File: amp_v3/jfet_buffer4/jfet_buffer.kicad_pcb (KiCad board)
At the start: 2 copper layers, 37.5 x 45.1 mm, 20 parts, among them J1 SIG_OUT_L1, J2 SIG_OUT_L1, J3 SIG_OUT_L1, J4 SIG_OUT_L2, Q1 2N5457, Q2 2N5457 DSG

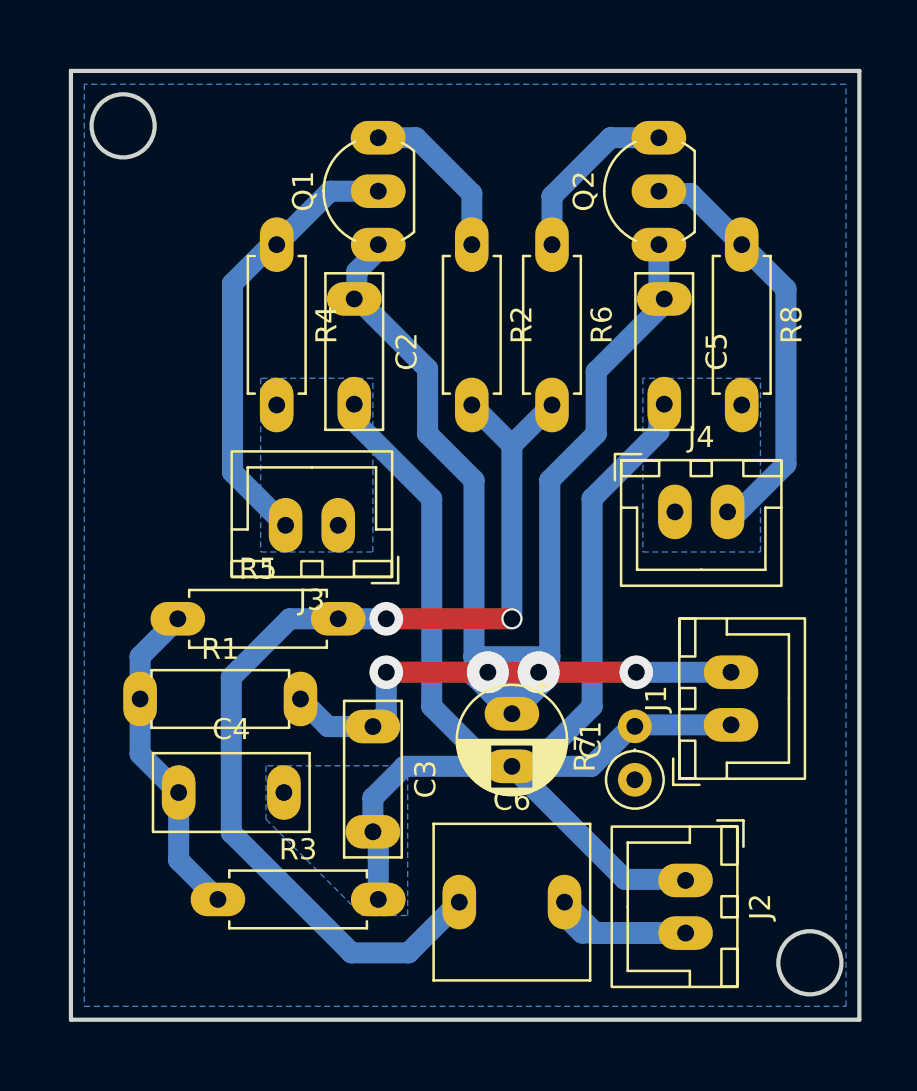
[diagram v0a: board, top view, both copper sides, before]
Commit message: update
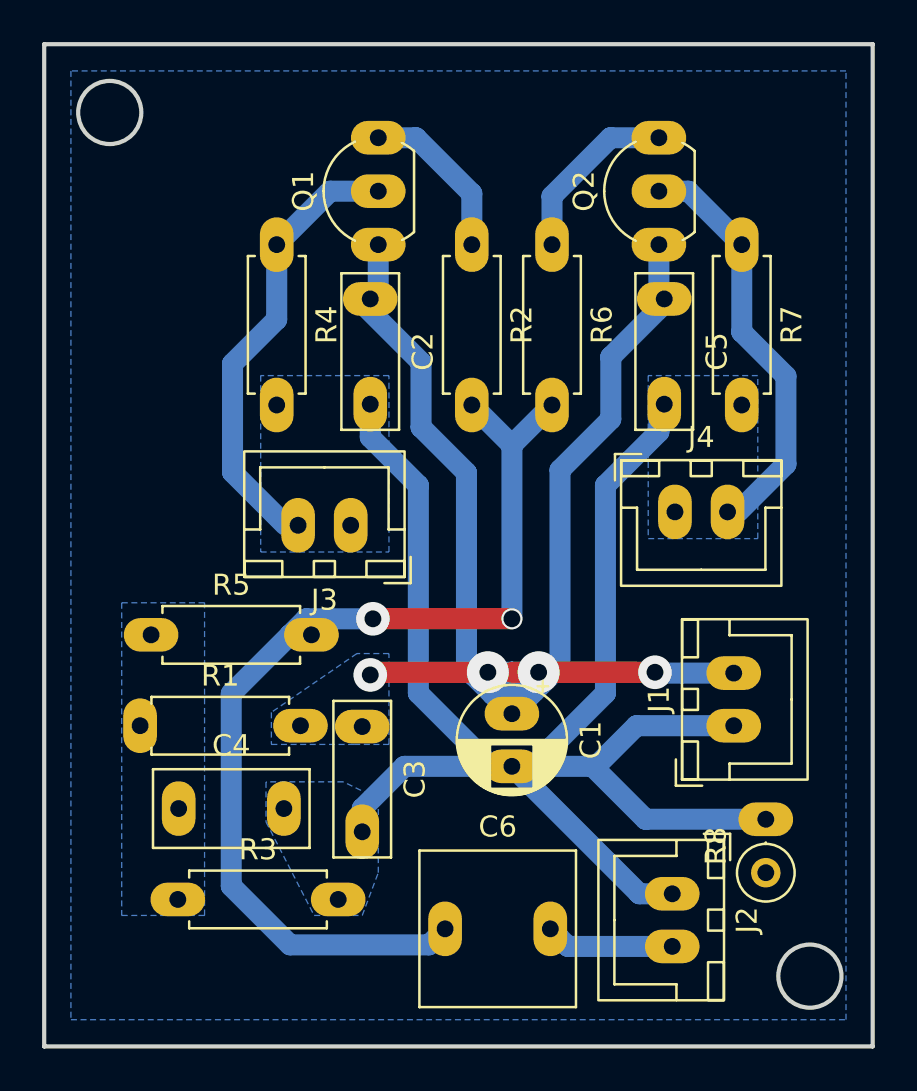
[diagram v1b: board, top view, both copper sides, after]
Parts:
- J1: value SIG_OUT_L1 -> PWR
- J2: value SIG_OUT_L1 -> INPUT
- J3: value SIG_OUT_L1 -> OUT1
- J4: value SIG_OUT_L2 -> OUT2
- Q2: value 2N5457 DSG -> 2N5457
- moved R8 7.63 mm to (103.9, 92.8)
- moved R3 1.91 mm to (75.9, 94.1)
- moved R5 1.48 mm to (74.6, 81.5)
- moved C6 1.44 mm to (88.6, 95.5)
- moved R1 1.27 mm to (74.1, 85.9)
- moved J2 0.90 mm to (99.4, 93.8)
- moved C2 0.76 mm to (85.1, 65.6)
- moved C4 0.76 mm to (76.0, 89.8)
- moved J3 0.59 mm to (84.1, 76.3)
- moved C3 0.51 mm to (84.7, 85.9)
- moved J1 0.13 mm to (102.3, 85.9)
- renumbered R8 to R7, R7 to R8
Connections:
- net /L_IN renamed /INPUT
- net /L_OUT_BUF1 renamed /OUT1
- net /L_OUT_BUF2 renamed /OUT2
- net /VBIAS_L renamed /VBIAS
- net /VBIAS_OUT_L renamed /VBIAS_OUT
- net GND_IN_L renamed GND
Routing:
- net /VBIAS: track 15.6 -> 0.00 mm
- net /INPUT: track 13.1 -> 6.14 mm
- net +20V: track 86.6 -> 82.6 mm
- net GND: track 76.1 -> 80.0 mm
- net /VBIAS_OUT: track 50.3 -> 51.3 mm
- added copper zone on B.Cu, net +20V
- added copper zone on B.Cu, net /VBIAS
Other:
- board size 37.5 x 45.1 mm -> 39.4 x 47.6 mm

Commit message: updates
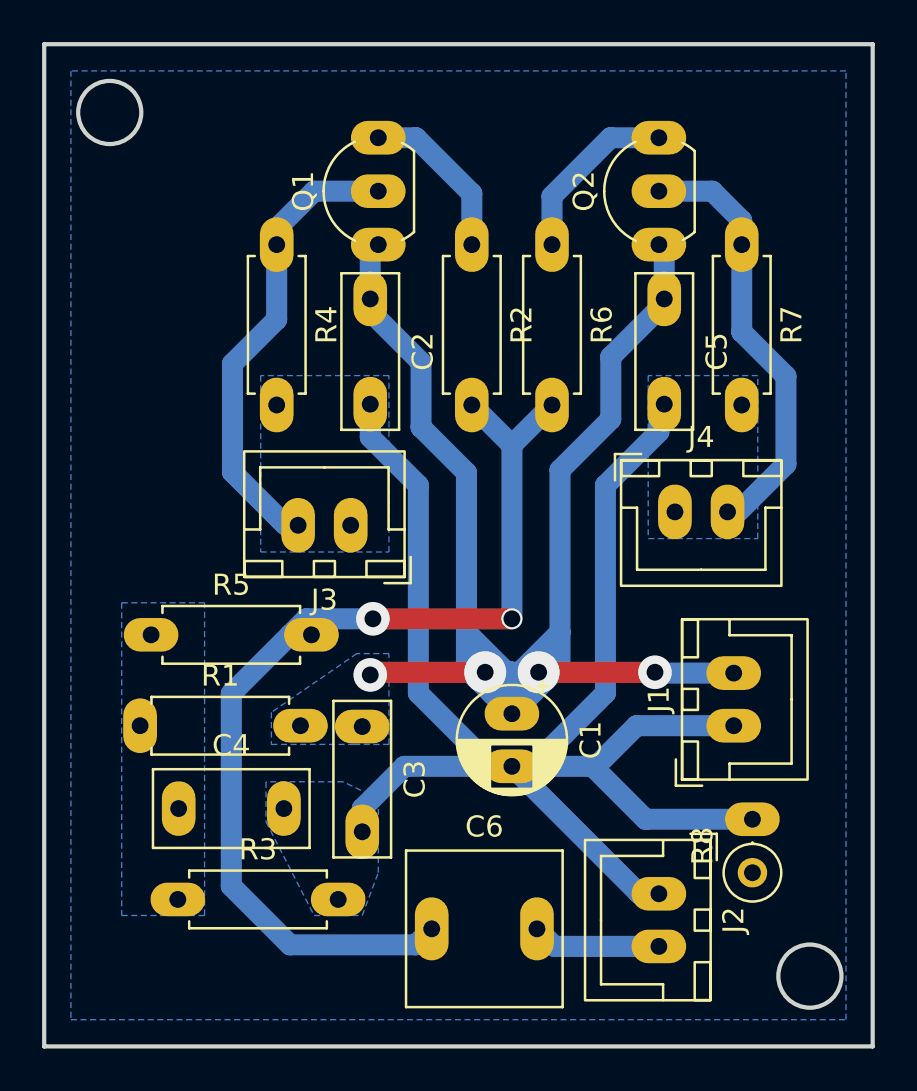
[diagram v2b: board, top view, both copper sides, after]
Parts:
- moved C6 0.64 mm to (88.0, 95.5)
- moved R8 0.64 mm to (103.2, 92.8)
- moved J2 0.63 mm to (98.8, 93.8)
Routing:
- net /VBIAS_OUT: track 51.3 -> 48.6 mm
- net +20V: track 82.6 -> 81.8 mm
- net /OUT2: track 19.5 -> 20.2 mm
- net GND: track 80.0 -> 79.4 mm
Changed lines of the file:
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@@
 	(footprint "Resistor_THT:R_Axial_DIN0207_L6.3mm_D2.5mm_P2.54mm_Vertical"
 		(layer "F.Cu")
-		(at 103.857 92.843 90)
+		(at 103.222 92.843 90)
 		(descr "Resistor, Axial_DIN0207 series, Axial, Vertical, pin pitch=2.54mm, 0.25W = 1/4W, length*diameter=6.3*2.5mm^2, http://cdn-reichelt.de/documents/datenblatt/B400/1_4W%23YAG.pdf")
 		(tags "Resistor Axial_DIN0207 series Axial Vertical pin pitch 2.54mm 0.25W = 1/4W length 6.3mm diameter 2.5mm")
@@
 		)
 		(pad "1" thru_hole oval
-			(at 0 0 270)
+			(at 0 0)
 			(size 1.6 2.6)
 			(drill 0.8)
@@
 		)
 		(pad "1" thru_hole oval
-			(at 0 0 270)
+			(at 0 0)
 			(size 1.6 2.6)
 			(drill 0.8)
@@
 	(footprint "Connector_JST:JST_XH_B2B-XH-A_1x02_P2.50mm_Vertical"
 		(layer "F.Cu")
-		(at 99.411776 93.844892 -90)
+		(at 98.777 93.844892 -90)
 		(descr "JST XH series connector, B2B-XH-A (http://www.jst-mfg.com/product/pdf/eng/eXH.pdf)")
 		(tags "connector JST XH vertical")
@@
 	(footprint "Capacitor_THT:C_Rect_L7.2mm_W7.2mm_P5.00mm_FKS2_FKP2_MKS2_MKP2"
 		(layer "F.Cu")
-		(at 88.617 95.51)
+		(at 87.982 95.51)
 		(descr "C, Rect series, Radial, pin pitch=5.00mm, length*width=7.2*7.2mm^2, Capacitor, http://www.wima.com/EN/WIMA_FKS_2.pdf")
 		(tags "C Rect series Radial pin pitch 5.00mm length 7.2mm width 7.2mm Capacitor")
@@
 		(pad "1" thru_hole oval
 			(at 0 0)
-			(size 1.6 2.6)
+			(size 1.6 3)
 			(drill 0.8)
 			(layers "*.Cu" "*.Mask")
@@
 		(pad "2" thru_hole oval
 			(at 5 0)
-			(size 1.6 2.6)
+			(size 1.6 3)
 			(drill 0.8)
 			(layers "*.Cu" "*.Mask")
@@
 	)
 	(segment
+		(start 97.849005 93.844892)
+		(end 91.792 87.787887)
+		(width 1)
+		(layer "B.Cu")
+		(net "GND")
+	)
+	(segment
 		(start 91.792 87.787887)
 		(end 95.782887 87.787887)
@@
 	)
 	(segment
+		(start 98.777 93.844892)
+		(end 97.849005 93.844892)
+		(width 1)
+		(layer "B.Cu")
+		(net "GND")
+	)
+	(segment
 		(start 86.687113 87.787887)
 		(end 91.792 87.787887)
@@
 	)
 	(segment
-		(start 97.849005 93.844892)
-		(end 91.792 87.787887)
-		(width 1)
-		(layer "B.Cu")
-		(net "GND")
-	)
-	(segment
 		(start 90.822152 87.787887)
 		(end 91.792 87.787887)
@@
 	)
 	(segment
-		(start 99.411776 93.844892)
-		(end 97.849005 93.844892)
-		(width 1)
-		(layer "B.Cu")
-		(net "GND")
-	)
-	(segment
 		(start 92.761848 87.787887)
 		(end 91.792 87.787887)
@@
 	)
 	(segment
-		(start 81.251 81.54)
-		(end 82.267 81.54)
+		(start 81.251 96.272)
+		(end 78.457 93.478)
 		(width 1)
 		(layer "B.Cu")
@@
 	)
 	(segment
-		(start 82.267 81.54)
-		(end 83.029 80.778)
+		(start 85.188 80.778)
+		(end 82.013 80.778)
 		(width 1)
 		(layer "B.Cu")
@@
 	)
 	(segment
-		(start 78.457 93.478)
-		(end 78.457 84.334)
+		(start 87.982 95.51)
+		(end 87.22 96.272)
 		(width 1)
 		(layer "B.Cu")
@@
 	)
 	(segment
-		(start 85.188 80.778)
-		(end 82.013 80.778)
+		(start 78.457 84.334)
+		(end 81.251 81.54)
 		(width 1)
 		(layer "B.Cu")
@@
 	)
 	(segment
-		(start 89.887 70.618)
-		(end 91.792 72.523)
+		(start 78.457 93.478)
+		(end 78.457 84.334)
 		(width 1)
 		(layer "B.Cu")
@@
 	)
 	(segment
-		(start 91.792 80.778)
+		(start 89.887 70.618)
 		(end 91.792 72.523)
 		(width 1)
@@
 	)
 	(segment
-		(start 88.617 95.51)
-		(end 87.855 96.272)
+		(start 91.792 80.778)
+		(end 91.792 72.523)
 		(width 1)
 		(layer "B.Cu")
@@
 	)
 	(segment
-		(start 87.855 96.272)
-		(end 81.251 96.272)
-		(width 1)
-		(layer "B.Cu")
-		(net "/VBIAS_OUT")
-	)
-	(segment
 		(start 82.013 80.778)
 		(end 81.251 81.54)
@@
 	)
 	(segment
-		(start 81.251 96.272)
-		(end 78.457 93.478)
+		(start 87.22 96.272)
+		(end 81.251 96.272)
 		(width 1)
 		(layer "B.Cu")
@@
 	)
 	(segment
-		(start 78.457 84.334)
-		(end 81.251 81.54)
+		(start 85.442 60.458)
+		(end 82.394 60.458)
 		(width 1)
 		(layer "B.Cu")
-		(net "/VBIAS_OUT")
+		(net "/OUT1")
 	)
 	(segment
@@
 	)
 	(segment
-		(start 85.442 60.458)
-		(end 83.156 60.458)
-		(width 1)
-		(layer "B.Cu")
-		(net "/OUT1")
-	)
-	(segment
 		(start 78.516 68.654)
 		(end 78.516 73.812)
@@
 	)
 	(segment
-		(start 83.156 60.458)
-		(end 80.616 62.998)
+		(start 82.394 60.458)
+		(end 80.616 62.236)
 		(width 1)
 		(layer "B.Cu")
@@
 		(net "+20V")
 	)
-	(segment
-		(start 97.702 83.318)
-		(end 91.792 83.318)
-		(width 1)
-		(layer "F.Cu")
-		(net "+20V")
-	)
 	(via
-		(at 90.649 83.318)
+		(at 90.522 83.318)
 		(size 2)
 		(drill 0.8)
@@
 	)
 	(segment
-		(start 89.633 73.833848)
+		(start 89.633 81.413)
 		(end 89.633 83.128887)
 		(width 1)
@@
 	)
 	(segment
-		(start 87.474 71.674848)
-		(end 89.633 73.833848)
+		(start 94.078 73.706848)
+		(end 94.078 81.413)
 		(width 1)
 		(layer "B.Cu")
@@
 	)
 	(segment
-		(start 98.777 62.998)
-		(end 98.777 66.046)
+		(start 87.474 71.674848)
+		(end 89.633 73.833848)
 		(width 1)
 		(layer "B.Cu")
@@
 	)
 	(segment
-		(start 85.442 65.197)
-		(end 85.061 65.578)
-		(width 1)
-		(layer "B.Cu")
-		(net "+20V")
-	)
-	(segment
 		(start 91.792 83.318)
-		(end 91.792 85.287887)
+		(end 91.792 83.953)
 		(width 1)
 		(layer "B.Cu")
@@
 	)
 	(segment
-		(start 94.078 73.706848)
+		(start 94.078 81.413)
 		(end 94.078 83.001887)
 		(width 1)
@@
 	)
 	(segment
+		(start 99.031 65.578)
+		(end 99.031 63.252)
+		(width 1)
+		(layer "B.Cu")
+		(net "+20V")
+	)
+	(segment
+		(start 91.792 83.572)
+		(end 91.919 83.572)
+		(width 1)
+		(layer "B.Cu")
+		(net "+20V")
+	)
+	(segment
 		(start 91.792 83.318)
 		(end 92.713444 84.239444)
@@
 	)
 	(segment
+		(start 85.061 65.578)
+		(end 85.061 63.379)
+		(width 1)
+		(layer "B.Cu")
+		(net "+20V")
+	)
+	(segment
 		(start 89.992 83.487887)
 		(end 90.870556 84.366444)
@@
 	)
 	(segment
+		(start 85.061 66.173)
+		(end 87.474 68.586)
+		(width 1)
+		(layer "B.Cu")
+		(net "+20V")
+	)
+	(segment
 		(start 96.491 71.293848)
 		(end 94.078 73.706848)
@@
 	)
 	(segment
+		(start 91.792 83.572)
+		(end 89.633 81.413)
+		(width 1)
+		(layer "B.Cu")
+		(net "+20V")
+	)
+	(segment
 		(start 98.777 66.046)
 		(end 96.491 68.332)
@@
 	)
 	(segment
+		(start 89.633 73.833848)
+		(end 89.633 81.413)
+		(width 1)
+		(layer "B.Cu")
+		(net "+20V")
+	)
+	(segment
 		(start 91.792 85.287887)
 		(end 94.078 83.001887)
@@
 	)
 	(segment
+		(start 91.792 83.953)
+		(end 91.792 85.287887)
+		(width 1)
+		(layer "B.Cu")
+		(net "+20V")
+	)
+	(segment
 		(start 91.792 83.318)
 		(end 90.870556 84.239444)
@@
 	)
 	(segment
-		(start 85.442 62.998)
-		(end 85.442 65.197)
+		(start 91.919 83.572)
+		(end 94.078 81.413)
 		(width 1)
 		(layer "B.Cu")
@@
 	)
 	(segment
-		(start 84.466 65.578)
-		(end 87.474 68.586)
+		(start 91.792 83.953)
+		(end 91.792 83.572)
 		(width 1)
 		(layer "B.Cu")
@@
 	)
 	(segment
+		(start 85.061 63.379)
+		(end 85.442 62.998)
+		(width 1)
+		(layer "B.Cu")
+		(net "+20V")
+	)
+	(segment
 		(start 91.792 83.318)
 		(end 90.161887 83.318)
@@
 	)
 	(segment
-		(start 98.777 60.458)
-		(end 100.174 60.458)
+		(start 102.714 61.855)
+		(end 102.714 62.998)
 		(width 1)
 		(layer "B.Cu")
@@
 	)
 	(segment
-		(start 104.814 73.431)
-		(end 102.547 75.698)
+		(start 101.317 60.458)
+		(end 102.714 61.855)
 		(width 1)
 		(layer "B.Cu")
@@
 	)
 	(segment
-		(start 102.714 62.998)
-		(end 102.714 67.148152)
+		(start 104.814 73.431)
+		(end 102.547 75.698)
 		(width 1)
 		(layer "B.Cu")
@@
 	)
 	(segment
-		(start 100.174 60.458)
-		(end 102.714 62.998)
+		(start 102.714 62.998)
+		(end 102.714 67.148152)
 		(width 1)
 		(layer "B.Cu")
@@
 	)
 	(segment
+		(start 98.777 60.458)
+		(end 101.317 60.458)
+		(width 1)
+		(layer "B.Cu")
+		(net "/OUT2")
+	)
+	(segment
 		(start 87.234 57.918)
 		(end 89.887 60.571)
@@
 	)
 	(segment
-		(start 99.411776 96.344892)
-		(end 94.451892 96.344892)
+		(start 93.816892 96.344892)
+		(end 92.982 95.51)
 		(width 1)
 		(layer "B.Cu")
@@
 	)
 	(segment
-		(start 94.451892 96.344892)
-		(end 93.617 95.51)
+		(start 98.777 96.344892)
+		(end 93.816892 96.344892)
 		(width 1)
 		(layer "B.Cu")
